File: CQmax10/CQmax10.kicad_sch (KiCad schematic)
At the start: 0 parts

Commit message: schematics
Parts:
- added J1, J2, J3, J4, J5, J6: ~, kicad8-2:Pmod_socket, symbol kicad8-2:Pmod_Socket
- added J7, J8: Conn_02x25_Odd_Even, Connector_PinSocket_2.54mm:PinSocket_2x25_P2.54mm_Vertical, symbol Connector_Generic:Conn_02x25_Odd_Even

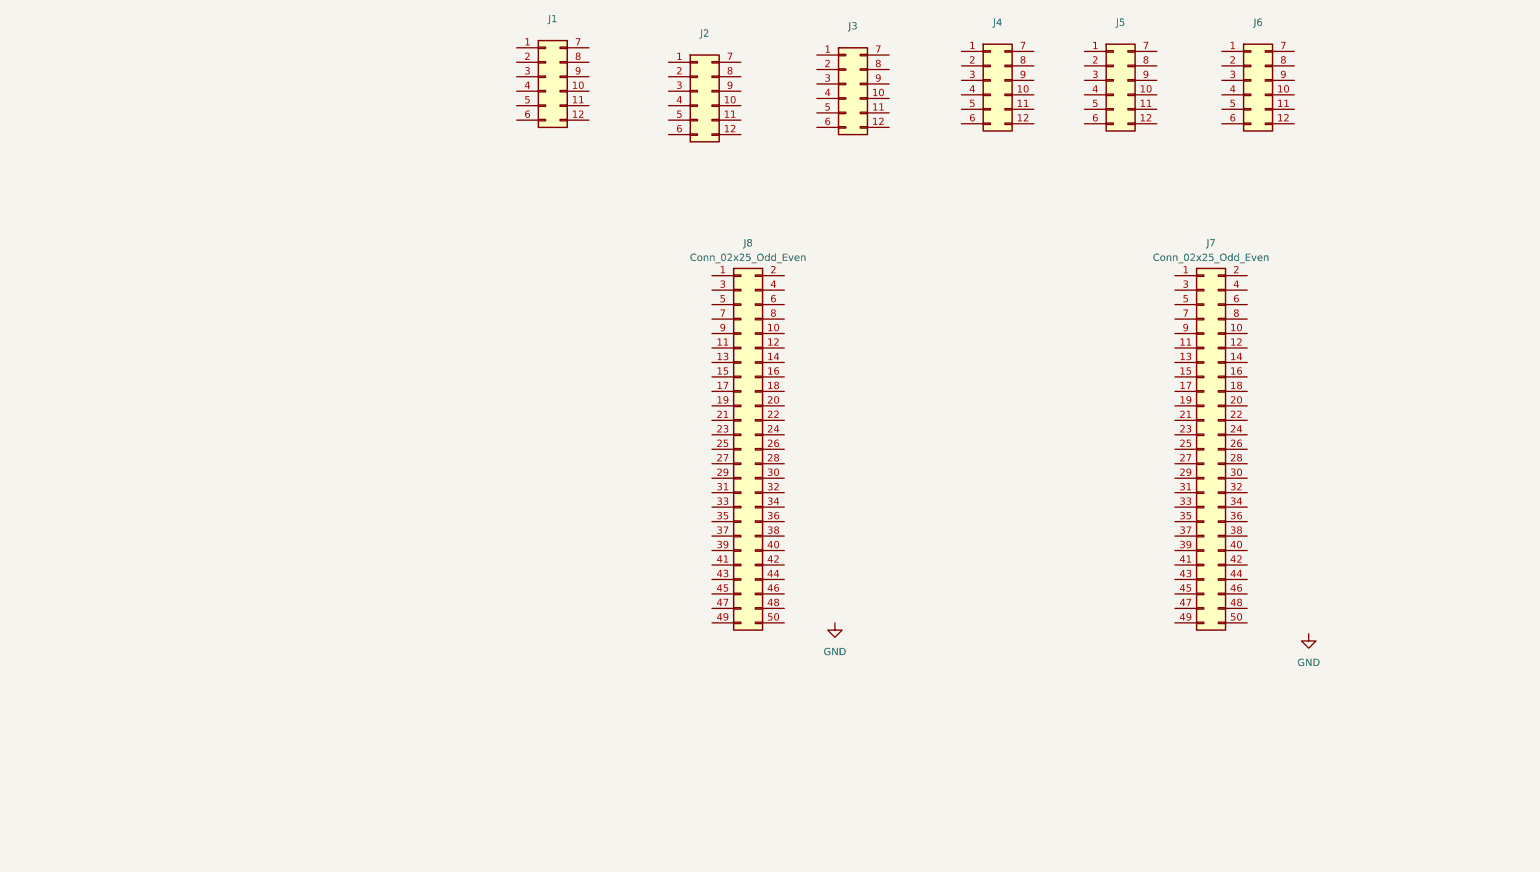
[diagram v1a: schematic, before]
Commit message: schematics
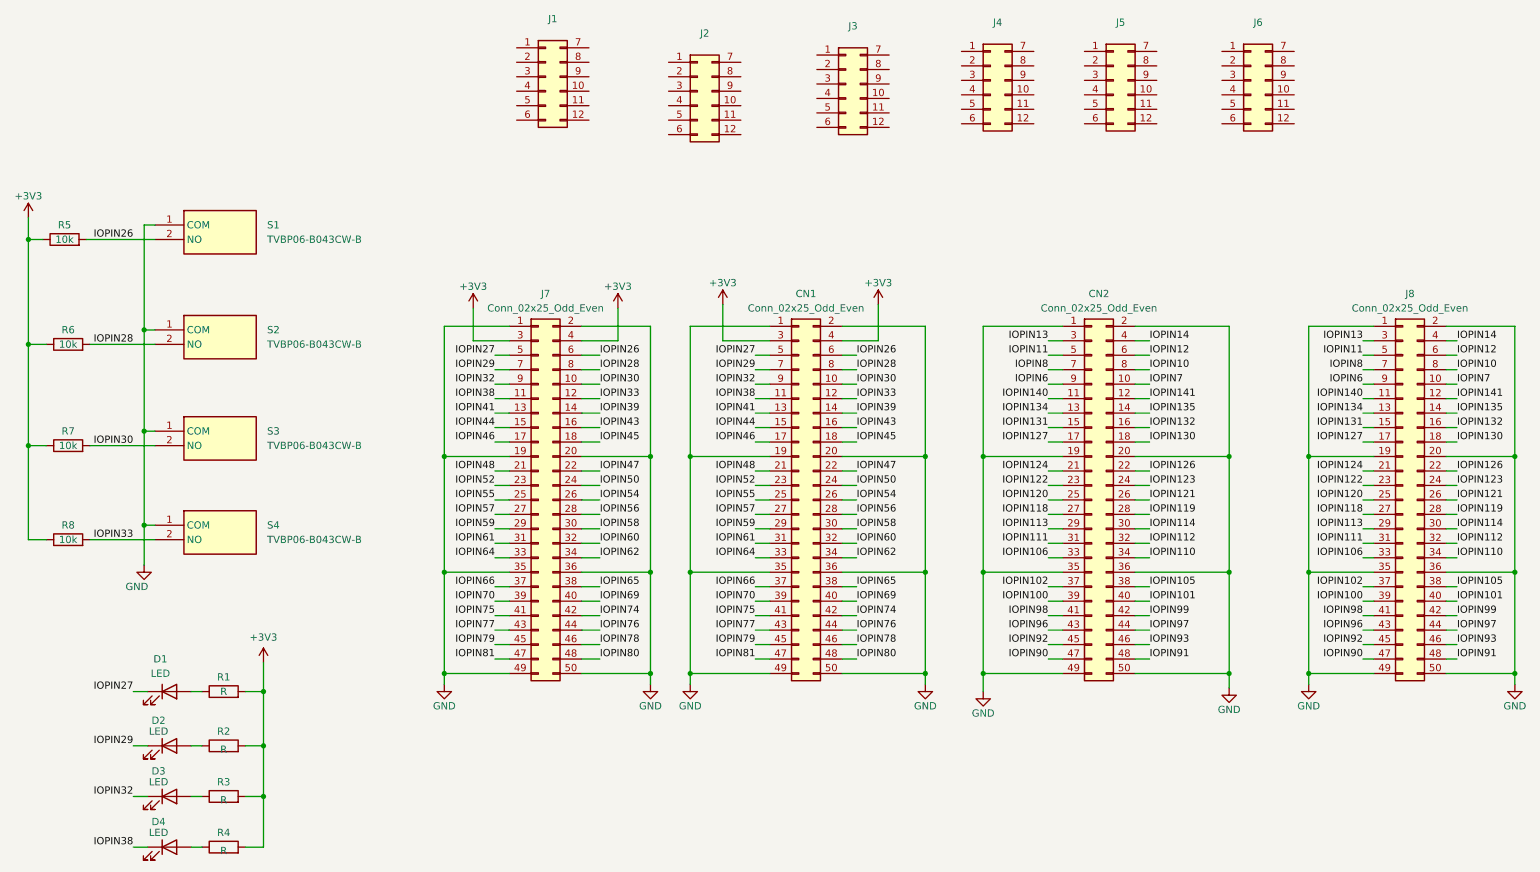
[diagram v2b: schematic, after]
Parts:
- added CN2: Conn_02x25_Odd_Even, Connector_PinSocket_2.54mm:PinSocket_2x25_P2.54mm_Vertical, symbol Connector_Generic:Conn_02x25_Odd_Even
- added D1, D2, D3, D4: LED, LED_SMD:LED_0603_1608Metric_Pad1.05x0.95mm_HandSolder, symbol Device:LED
- added J7: Conn_02x25_Odd_Even, Connector_PinHeader_2.54mm:PinHeader_2x25_P2.54mm_Vertical, symbol Connector_Generic:Conn_02x25_Odd_Even
- added R1, R2, R3, R4: R, Resistor_SMD:R_0603_1608Metric_Pad0.98x0.95mm_HandSolder, symbol Device:R
- added R5, R6, R7, R8: 10k, Resistor_SMD:R_0603_1608Metric_Pad0.98x0.95mm_HandSolder, symbol Device:R
- added S1, S2, S3, S4: TVBP06-B043CW-B, TVBP06B043CWB, symbol kicad8:TVBP06-B043CW-B
- J8: footprint Connector_PinSocket_2.54mm:PinSocket_2x25_P2.54mm_Vertical -> Connector_PinHeader_2.54mm:PinHeader_2x25_P2.54mm_Vertical
- renumbered J7 to CN1
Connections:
- net GND: now also CN1.1 (Pin_1), CN1.19 (Pin_19), CN1.2 (Pin_2), CN1.20 (Pin_20), CN1.35 (Pin_35), CN1.36 (Pin_36), CN1.49 (Pin_49), CN1.50 (Pin_50), J8.1 (Pin_1), J8.19 (Pin_19), J8.2 (Pin_2), J8.20 (Pin_20), J8.35 (Pin_35), J8.36 (Pin_36), J8.49 (Pin_49), J8.50 (Pin_50), CN2.1 (Pin_1), CN2.19 (Pin_19), CN2.2 (Pin_2), CN2.20 (Pin_20), CN2.35 (Pin_35), CN2.36 (Pin_36), CN2.49 (Pin_49), CN2.50 (Pin_50), J7.1 (Pin_1), J7.19 (Pin_19), J7.2 (Pin_2), J7.20 (Pin_20), J7.35 (Pin_35), J7.36 (Pin_36), J7.49 (Pin_49), J7.50 (Pin_50), S1.1 (COM), S2.1 (COM), S3.1 (COM), S4.1 (COM)
- net IOPIN7: now reaches J8.10 (Pin_10)
- net IOPIN7: now also CN2.10 (Pin_10)
- net IOPIN140: now reaches J8.11 (Pin_11)
- net IOPIN140: now also CN2.11 (Pin_11)
- net IOPIN141: now reaches J8.12 (Pin_12)
- net IOPIN141: now also CN2.12 (Pin_12)
- net IOPIN134: now reaches J8.13 (Pin_13)
- net IOPIN134: now also CN2.13 (Pin_13)
- net IOPIN135: now reaches J8.14 (Pin_14)
- net IOPIN135: now also CN2.14 (Pin_14)
- net IOPIN131: now reaches J8.15 (Pin_15)
- net IOPIN131: now also CN2.15 (Pin_15)
- net IOPIN132: now reaches J8.16 (Pin_16)
- net IOPIN132: now also CN2.16 (Pin_16)
- net IOPIN127: now reaches J8.17 (Pin_17)
- net IOPIN127: now also CN2.17 (Pin_17)
- net IOPIN130: now reaches J8.18 (Pin_18)
- net IOPIN130: now also CN2.18 (Pin_18)
- net IOPIN124: now reaches J8.21 (Pin_21)
- net IOPIN124: now also CN2.21 (Pin_21)
- net IOPIN126: now reaches J8.22 (Pin_22)
- net IOPIN126: now also CN2.22 (Pin_22)
- net IOPIN122: now reaches J8.23 (Pin_23)
- net IOPIN122: now also CN2.23 (Pin_23)
- net IOPIN123: now reaches J8.24 (Pin_24)
- net IOPIN123: now also CN2.24 (Pin_24)
- net IOPIN120: now reaches J8.25 (Pin_25)
- net IOPIN120: now also CN2.25 (Pin_25)
- net IOPIN121: now reaches J8.26 (Pin_26)
- net IOPIN121: now also CN2.26 (Pin_26)
- net IOPIN118: now reaches J8.27 (Pin_27)
- net IOPIN118: now also CN2.27 (Pin_27)
- net IOPIN119: now reaches J8.28 (Pin_28)
- net IOPIN119: now also CN2.28 (Pin_28)
- net IOPIN113: now reaches J8.29 (Pin_29)
- net IOPIN113: now also CN2.29 (Pin_29)
- net IOPIN13: now reaches J8.3 (Pin_3)
- net IOPIN13: now also CN2.3 (Pin_3)
- net IOPIN114: now reaches J8.30 (Pin_30)
- net IOPIN114: now also CN2.30 (Pin_30)
- net IOPIN111: now reaches J8.31 (Pin_31)
- net IOPIN111: now also CN2.31 (Pin_31)
- net IOPIN112: now reaches J8.32 (Pin_32)
- net IOPIN112: now also CN2.32 (Pin_32)
- net IOPIN106: now reaches J8.33 (Pin_33)
- net IOPIN106: now also CN2.33 (Pin_33)
- net IOPIN110: now reaches J8.34 (Pin_34)
- net IOPIN110: now also CN2.34 (Pin_34)
- net IOPIN102: now reaches J8.37 (Pin_37)
- net IOPIN102: now also CN2.37 (Pin_37)
- net IOPIN105: now reaches J8.38 (Pin_38)
- net IOPIN105: now also CN2.38 (Pin_38)
- net IOPIN100: now reaches J8.39 (Pin_39)
- net IOPIN100: now also CN2.39 (Pin_39)
- net IOPIN14: now reaches J8.4 (Pin_4)
- net IOPIN14: now also CN2.4 (Pin_4)
- net IOPIN101: now reaches J8.40 (Pin_40)
- net IOPIN101: now also CN2.40 (Pin_40)
- net IOPIN98: now reaches J8.41 (Pin_41)
- net IOPIN98: now also CN2.41 (Pin_41)
- net IOPIN99: now reaches J8.42 (Pin_42)
- net IOPIN99: now also CN2.42 (Pin_42)
- net IOPIN96: now reaches J8.43 (Pin_43)
- net IOPIN96: now also CN2.43 (Pin_43)
- net IOPIN97: now reaches J8.44 (Pin_44)
- net IOPIN97: now also CN2.44 (Pin_44)
- net IOPIN92: now reaches J8.45 (Pin_45)
- net IOPIN92: now also CN2.45 (Pin_45)
- net IOPIN93: now reaches J8.46 (Pin_46)
- net IOPIN93: now also CN2.46 (Pin_46)
- net IOPIN90: now reaches J8.47 (Pin_47)
- net IOPIN90: now also CN2.47 (Pin_47)
- net IOPIN91: now reaches J8.48 (Pin_48)
- net IOPIN91: now also CN2.48 (Pin_48)
- net IOPIN11: now reaches J8.5 (Pin_5)
- net IOPIN11: now also CN2.5 (Pin_5)
- net IOPIN12: now reaches J8.6 (Pin_6)
- net IOPIN12: now also CN2.6 (Pin_6)
- net IOPIN8: now reaches J8.7 (Pin_7)
- net IOPIN8: now also CN2.7 (Pin_7)
- net IOPIN10: now reaches J8.8 (Pin_8)
- net IOPIN10: now also CN2.8 (Pin_8)
- net IOPIN6: now reaches J8.9 (Pin_9)
- net IOPIN6: now also CN2.9 (Pin_9)
- net IOPIN30: now reaches CN1.10 (Pin_10)
- net IOPIN30: now also J7.10 (Pin_10), R7.2, S3.2 (NO)
- net IOPIN38: now reaches CN1.11 (Pin_11)
- net IOPIN38: now also D4.1 (K), J7.11 (Pin_11)
- net IOPIN33: now reaches CN1.12 (Pin_12)
- net IOPIN33: now also J7.12 (Pin_12), R8.2, S4.2 (NO)
- net IOPIN41: now reaches CN1.13 (Pin_13)
- net IOPIN41: now also J7.13 (Pin_13)
- net IOPIN39: now reaches CN1.14 (Pin_14)
- net IOPIN39: now also J7.14 (Pin_14)
- net IOPIN44: now reaches CN1.15 (Pin_15)
- net IOPIN44: now also J7.15 (Pin_15)
- net IOPIN43: now reaches CN1.16 (Pin_16)
- net IOPIN43: now also J7.16 (Pin_16)
- net IOPIN46: now reaches CN1.17 (Pin_17)
- net IOPIN46: now also J7.17 (Pin_17)
- net IOPIN45: now reaches CN1.18 (Pin_18)
- net IOPIN45: now also J7.18 (Pin_18)
- net IOPIN48: now reaches CN1.21 (Pin_21)
- net IOPIN48: now also J7.21 (Pin_21)
- net IOPIN47: now reaches CN1.22 (Pin_22)
- net IOPIN47: now also J7.22 (Pin_22)
- net IOPIN52: now reaches CN1.23 (Pin_23)
- net IOPIN52: now also J7.23 (Pin_23)
- net IOPIN50: now reaches CN1.24 (Pin_24)
- net IOPIN50: now also J7.24 (Pin_24)
- net IOPIN55: now reaches CN1.25 (Pin_25)
- net IOPIN55: now also J7.25 (Pin_25)
- net IOPIN54: now reaches CN1.26 (Pin_26)
- net IOPIN54: now also J7.26 (Pin_26)
- net IOPIN57: now reaches CN1.27 (Pin_27)
- net IOPIN57: now also J7.27 (Pin_27)
- net IOPIN56: now reaches CN1.28 (Pin_28)
- net IOPIN56: now also J7.28 (Pin_28)
- net IOPIN59: now reaches CN1.29 (Pin_29)
- net IOPIN59: now also J7.29 (Pin_29)
- net +3V3: now reaches CN1.3 (Pin_3)
- net +3V3: now also CN1.4 (Pin_4), J7.3 (Pin_3), J7.4 (Pin_4), R1.2, R2.2, R3.2, R4.2, R5.1, R6.1, R7.1, R8.1
- net IOPIN58: now reaches CN1.30 (Pin_30)
- net IOPIN58: now also J7.30 (Pin_30)
- net IOPIN61: now reaches CN1.31 (Pin_31)
- net IOPIN61: now also J7.31 (Pin_31)
- net IOPIN60: now reaches CN1.32 (Pin_32)
- net IOPIN60: now also J7.32 (Pin_32)
- net IOPIN64: now reaches CN1.33 (Pin_33)
- net IOPIN64: now also J7.33 (Pin_33)
- net IOPIN62: now reaches CN1.34 (Pin_34)
- net IOPIN62: now also J7.34 (Pin_34)
- net IOPIN66: now reaches CN1.37 (Pin_37)
- net IOPIN66: now also J7.37 (Pin_37)
- net IOPIN65: now reaches CN1.38 (Pin_38)
- net IOPIN65: now also J7.38 (Pin_38)
- net IOPIN70: now reaches CN1.39 (Pin_39)
- net IOPIN70: now also J7.39 (Pin_39)
- net IOPIN69: now reaches CN1.40 (Pin_40)
- net IOPIN69: now also J7.40 (Pin_40)
- net IOPIN75: now reaches CN1.41 (Pin_41)
- net IOPIN75: now also J7.41 (Pin_41)
- net IOPIN74: now reaches CN1.42 (Pin_42)
- net IOPIN74: now also J7.42 (Pin_42)
- net IOPIN77: now reaches CN1.43 (Pin_43)
- net IOPIN77: now also J7.43 (Pin_43)
- net IOPIN76: now reaches CN1.44 (Pin_44)
- net IOPIN76: now also J7.44 (Pin_44)
- net IOPIN79: now reaches CN1.45 (Pin_45)
- net IOPIN79: now also J7.45 (Pin_45)
- net IOPIN78: now reaches CN1.46 (Pin_46)
- net IOPIN78: now also J7.46 (Pin_46)
- net IOPIN81: now reaches CN1.47 (Pin_47)
- net IOPIN81: now also J7.47 (Pin_47)
- net IOPIN80: now reaches CN1.48 (Pin_48)
- net IOPIN80: now also J7.48 (Pin_48)
- net IOPIN27: now reaches CN1.5 (Pin_5)
- net IOPIN27: now also D1.1 (K), J7.5 (Pin_5)
- net IOPIN26: now reaches CN1.6 (Pin_6)
- net IOPIN26: now also J7.6 (Pin_6), R5.2, S1.2 (NO)
- net IOPIN29: now reaches CN1.7 (Pin_7)
- net IOPIN29: now also D2.1 (K), J7.7 (Pin_7)
- net IOPIN28: now reaches CN1.8 (Pin_8)
- net IOPIN28: now also J7.8 (Pin_8), R6.2, S2.2 (NO)
- net IOPIN32: now reaches CN1.9 (Pin_9)
- net IOPIN32: now also D3.1 (K), J7.9 (Pin_9)
- new net: D4.2 (A), R4.1
- new net: D3.2 (A), R3.1
- new net: D1.2 (A), R1.1
- new net: D2.2 (A), R2.1
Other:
- moved on the sheet: CN1
